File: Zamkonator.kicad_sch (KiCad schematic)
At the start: 33 parts, among them J1 Screw_Terminal_01x06, J2 Micro_SD_Card_Det1, J3 Conn_01x08_Male, J5 Conn_01x04_Female, J6 Conn_01x03_Female

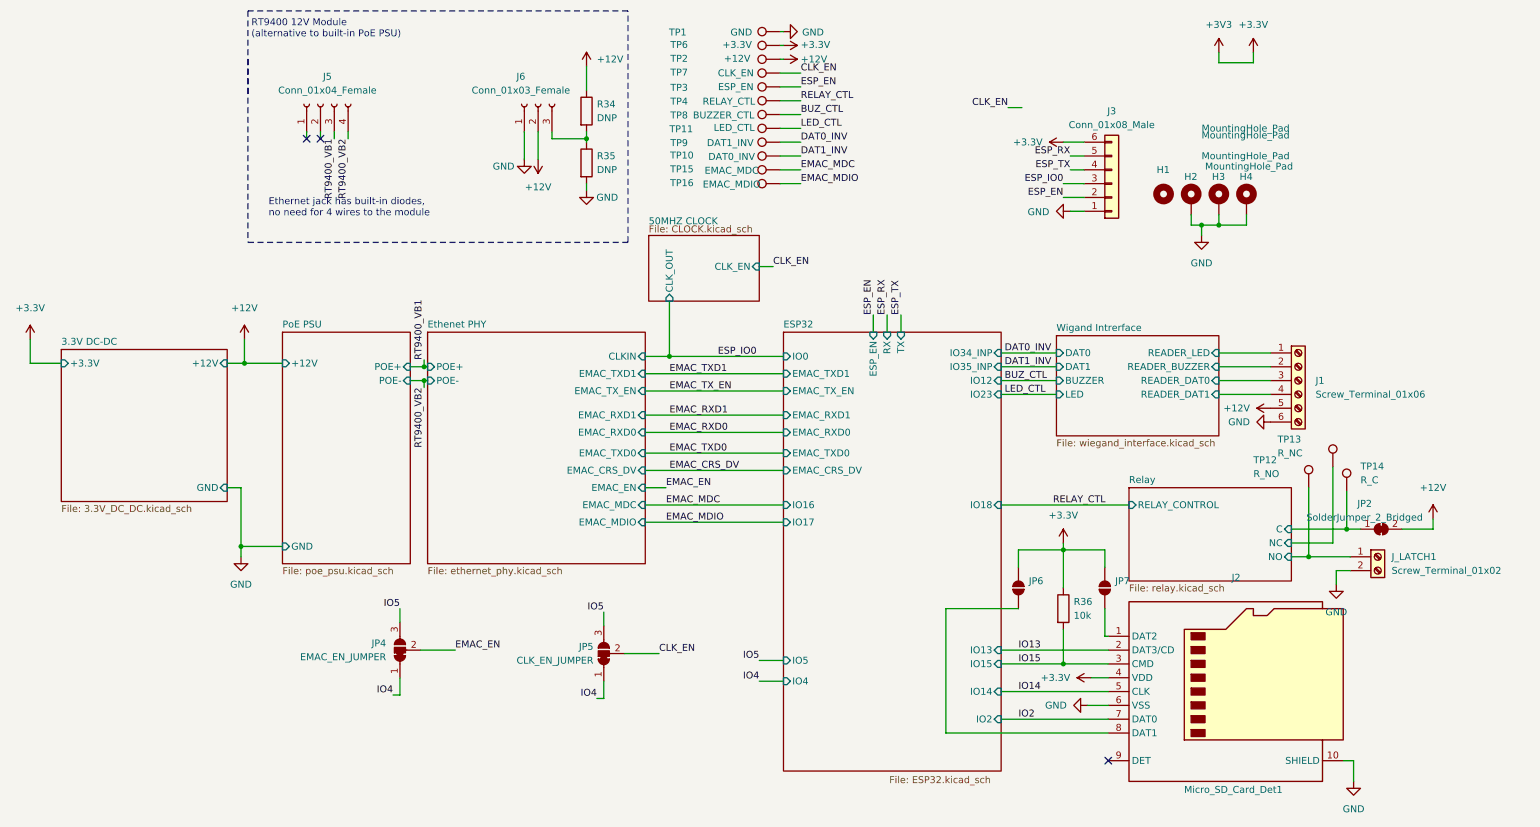
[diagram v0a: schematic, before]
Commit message: BOM updates & schematic fixes
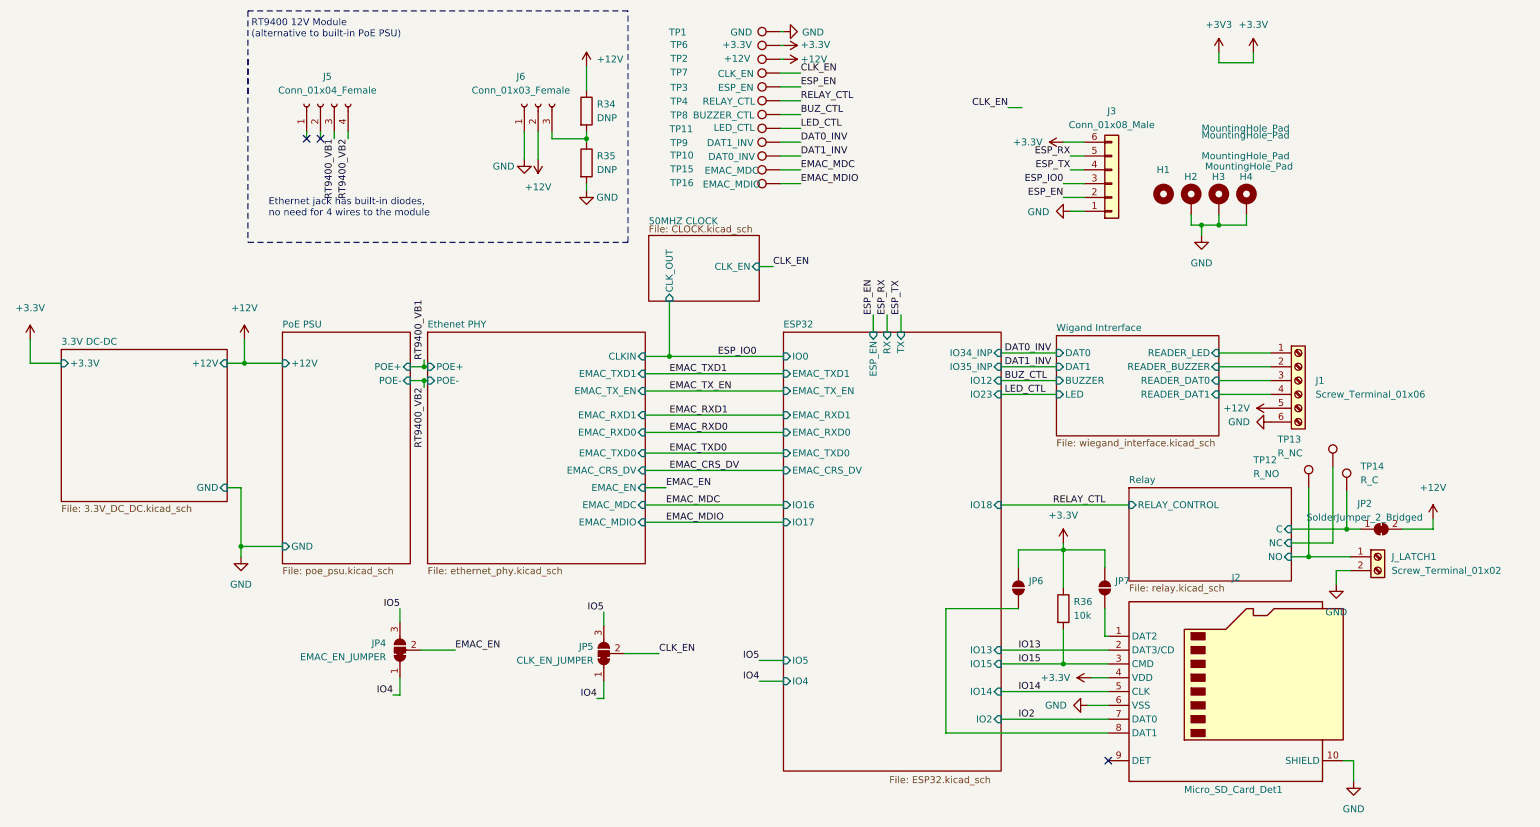
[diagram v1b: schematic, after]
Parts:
- TP1, TP10, TP11, TP15, TP16, TP2, TP3, TP4, TP6, TP7, TP8, TP9: now left out of the parts list
